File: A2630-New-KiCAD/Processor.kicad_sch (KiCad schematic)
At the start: 69 parts, among them U200 MC68030FE, U201 MC68882, U204 74HCT04, X1 25MHz, X2 25MHz

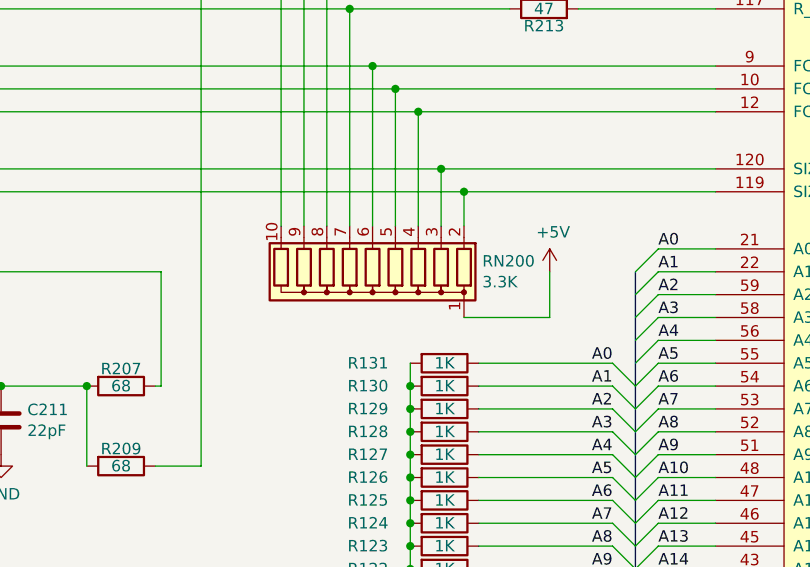
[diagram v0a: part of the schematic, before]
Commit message: Add files via upload
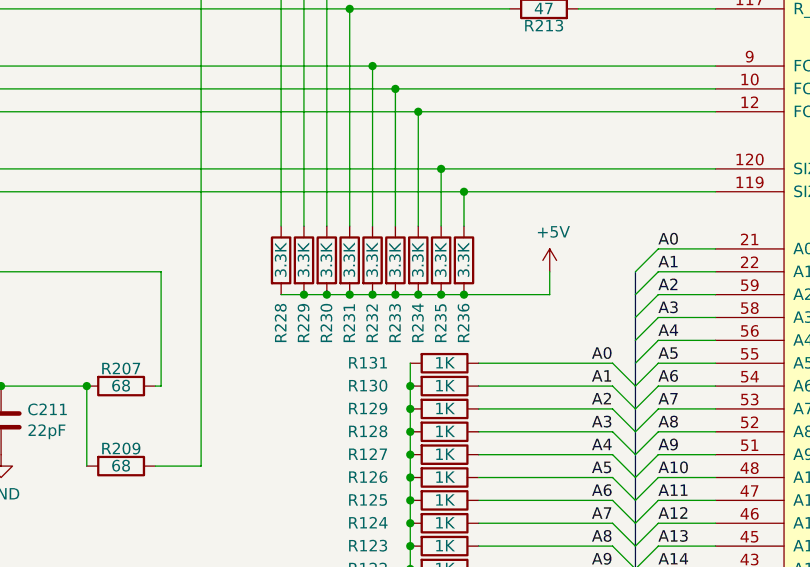
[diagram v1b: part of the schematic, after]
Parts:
- removed RN200: 3.3K, Resistor_THT:R_Array_SIP10, symbol Device:R_Network09
- added R228, R229, R230, R231, R232, R233, R234, R235, R236: 3.3K, Resistor_SMD:R_0805_2012Metric, symbol Device:R
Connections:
- net +5V: now also R228.2, R229.2, R230.2, R231.2, R232.2, R233.2, R234.2, R235.2, R236.2
- net FC0: now also R234.1
- net FC1: now also R233.1
- net FC2: now also R232.1
- net R_W: now also R231.1
- net SIZ0: now also R236.1
- net SIZ1: now also R235.1
- net _AS: now also R230.1
- net _CPURESET: now also R228.1
- net _DS: now also R229.1
